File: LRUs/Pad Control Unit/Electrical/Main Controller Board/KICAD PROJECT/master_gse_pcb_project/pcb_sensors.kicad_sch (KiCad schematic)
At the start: 10 parts, among them U15 TMP102xxDRL, U16 TMP102xxDRL

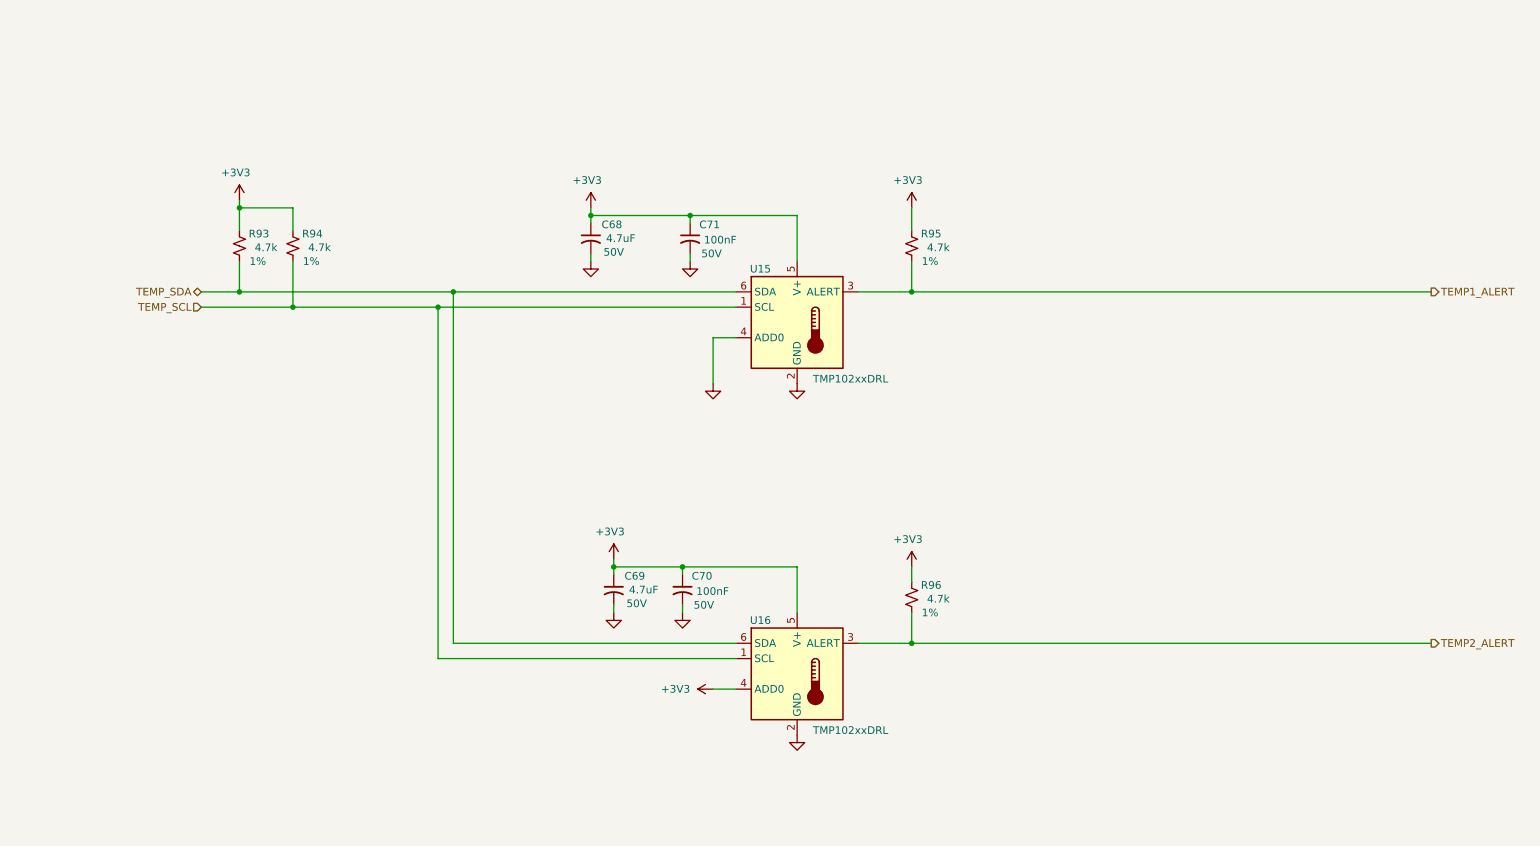
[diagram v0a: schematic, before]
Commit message: Committ latest changes
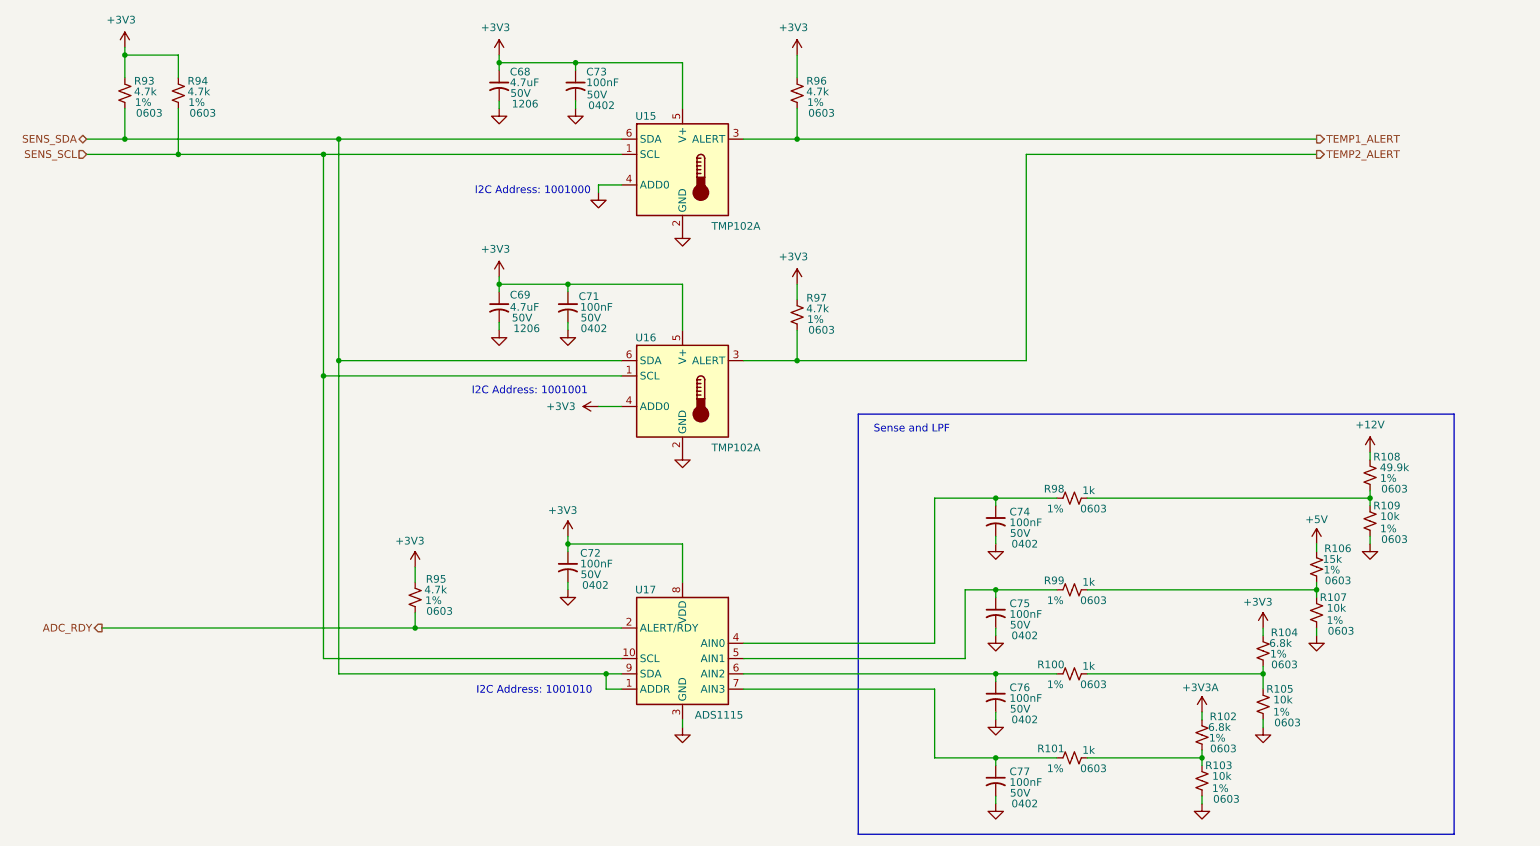
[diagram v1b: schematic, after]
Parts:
- added C72, C74, C75, C76, C77: 100nF, Capacitor_SMD:C_0402_1005Metric, symbol Device:C_Small_US
- added R100, R101, R98, R99: 1k, Resistor_SMD:R_0603_1608Metric, symbol Device:R_Small_US
- added R102, R104: 6.8k, Resistor_SMD:R_0603_1608Metric, symbol Device:R_Small_US
- added R103, R105, R107, R109: 10k, Resistor_SMD:R_0603_1608Metric, symbol Device:R_Small_US
- added R106: 15k, Resistor_SMD:R_0603_1608Metric, symbol Device:R_Small_US
- added R108: 49.9k, Resistor_SMD:R_0603_1608Metric, symbol Device:R_Small_US
- added R95: 4.7k, Resistor_SMD:R_0603_1608Metric, symbol Device:R_Small_US
- added U17: ADS1115, Package_SO:TSSOP-10_3x3mm_P0.5mm, symbol Analog_ADC:ADS1115IDGS
- C68, C69: Footprint_Size (none) -> 1206
- C71: renamed from C70; Footprint_Size (none) -> 0402
- C73: renamed from C71; Footprint_Size (none) -> 0402
- R93, R94: Footprint_Size (none) -> 0603
- R96: renamed from R95; Footprint_Size (none) -> 0603
- R97: renamed from R96; Footprint_Size (none) -> 0603
- U15, U16: value TMP102xxDRL -> TMP102A
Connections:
- net +3V3: now also C72.1, R104.2, R95.2, U17.8 (VDD)
- net GND: now also C72.2, C74.2, C75.2, C76.2, C77.2, R103.2, R105.2, R107.2, R109.2, U17.3 (GND)
- net TEMP_SCL renamed SENS_SCL
- net SENS_SCL: now also U17.10 (SCL)
- net TEMP_SDA renamed SENS_SDA
- net SENS_SDA: now also U17.1 (ADDR), U17.9 (SDA)
- new net: R108.2, R109.1, R98.1
- new net: C75.1, R99.2, U17.5 (AIN1)
- new net: R106.1, R107.1, R99.1
- new net: C77.1, R101.2, U17.7 (AIN3)
- new net: R100.1, R104.1, R105.1
- new net: C76.1, R100.2, U17.6 (AIN2)
- new net: C74.1, R98.2, U17.4 (AIN0)
- new net: R101.1, R102.1, R103.1
- new net +12V: R108.1
- new net +3V3A: R102.2
- new net +5V: R106.2
- new net ADC_RDY: R95.1, U17.2 (ALERT/RDY)
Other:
- note added: "I2C Address: 1001000"
- note added: "I2C Address: 1001001"
- note added: "I2C Address: 1001010"
- note added: "Sense and LPF"
- moved on the sheet: C68, C69, C71, C73, R93, R94, R96, R97, U15, U16
